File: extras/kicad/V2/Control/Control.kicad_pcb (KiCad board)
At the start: 2 copper layers, 181.3 x 110 mm, 45 parts, among them J1 Ultrasonic Ranging, J2 Conn_01x05, J3 Output, J4 Input, J6 left, J7 right, P8 BeagleBone_Black_Header, P9 BeagleBone_Black_Header, U1 SparkFun-micromod, U2 MPU-6050, U4 BNO085-breackout, U5 TJA1042T-3, U6 PCA9557PW

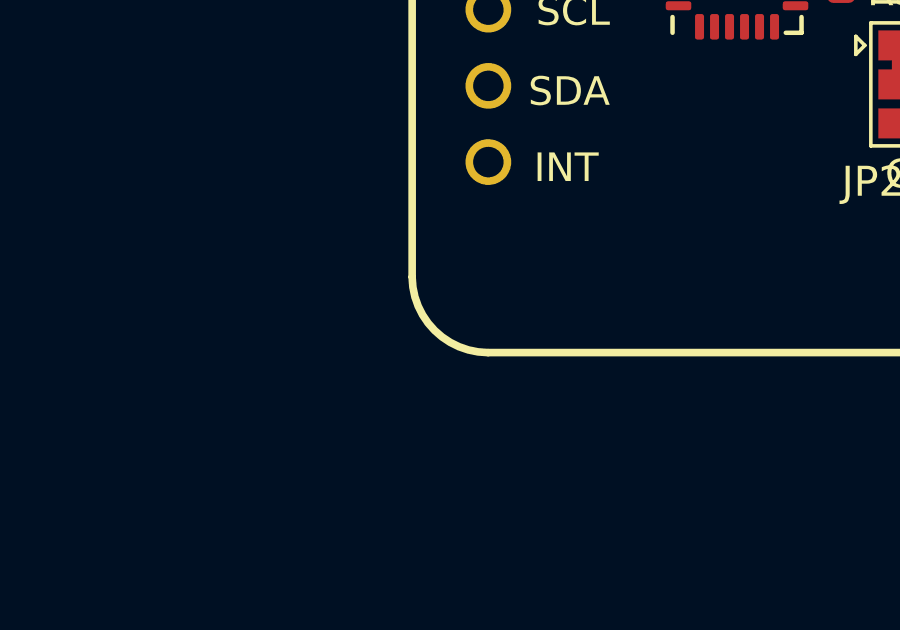
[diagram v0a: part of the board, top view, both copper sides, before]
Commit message: f
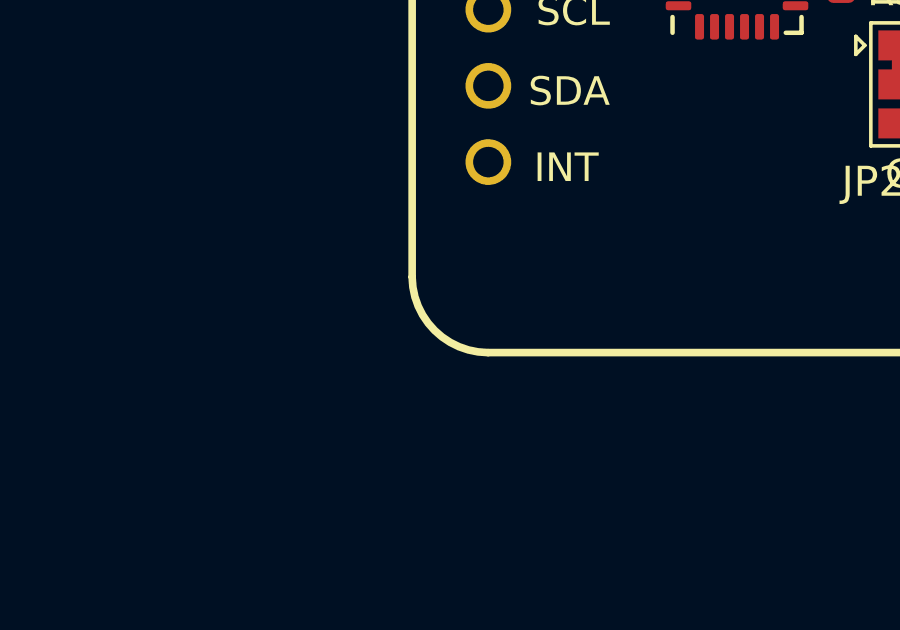
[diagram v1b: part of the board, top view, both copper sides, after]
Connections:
- J6 pad 21: +3V3 -> GND
- J6 pad 33: +3V3 -> GND
- J7 pad 32: +3V3 -> GND
- J7 pad 40: +3V3 -> GND
- P9 pad 17: /GPIO[4] -> SPI_CS
- U1 pad 55: SCL -> SPI_CS
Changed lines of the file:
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@@
   (net 169 "/GPIO[48]")
   (net 170 "/GPIO[51]")
-  (net 171 "/GPIO[4]")
+  (net 171 "SPI_CS")
   (net 172 "/GPIO[5]")
   (net 173 "unconnected-(U6-Pad10)")
@@
       (net 17 "/yellow_1") (pinfunction "AUD_IN") (pintype "input"))
     (pad "55" smd rect (at 4.25 -3.97) (size 0.3 2) (layers "F.Cu" "F.Paste" "F.Mask")
-      (net 2 "SCL") (pinfunction "SPI_CS") (pintype "input"))
+      (net 171 "SPI_CS") (pinfunction "SPI_CS") (pintype "input"))
     (pad "56" smd rect (at 4.5 3.98) (size 0.3 2) (layers "F.Cu" "F.Paste" "F.Mask")
       (net 19 "/Green_1") (pinfunction "AUD_OUT") (pintype "input"))
@@
       (net 1 "GND") (pinfunction "Pin_20") (pintype "passive"))
     (pad "21" thru_hole oval (at 0 25.4 90) (size 1.7 1.7) (drill 1) (layers F&B.Cu *.Mask)
-      (net 4 "+3V3") (pinfunction "Pin_21") (pintype "passive"))
+      (net 1 "GND") (pinfunction "Pin_21") (pintype "passive"))
     (pad "22" thru_hole oval (at 2.54 25.4 90) (size 1.7 1.7) (drill 1) (layers F&B.Cu *.Mask)
       (net 14 "unconnected-(J6-Pad22)") (pinfunction "Pin_22") (pintype "passive"))
@@
       (net 1 "GND") (pinfunction "Pin_32") (pintype "passive"))
     (pad "33" thru_hole oval (at 0 40.64 90) (size 1.7 1.7) (drill 1) (layers F&B.Cu *.Mask)
-      (net 4 "+3V3") (pinfunction "Pin_33") (pintype "passive"))
+      (net 1 "GND") (pinfunction "Pin_33") (pintype "passive"))
     (pad "34" thru_hole oval (at 2.54 40.64 90) (size 1.7 1.7) (drill 1) (layers F&B.Cu *.Mask)
       (net 23 "BIN1_1") (pinfunction "Pin_34") (pintype "passive"))
@@
       (net 1 "GND") (pinfunction "Pin_31") (pintype "passive"))
     (pad "32" thru_hole oval (at 2.54 38.1 90) (size 1.7 1.7) (drill 1) (layers F&B.Cu *.Mask)
-      (net 4 "+3V3") (pinfunction "Pin_32") (pintype "passive"))
+      (net 1 "GND") (pinfunction "Pin_32") (pintype "passive"))
     (pad "33" thru_hole oval (at 0 40.64 90) (size 1.7 1.7) (drill 1) (layers F&B.Cu *.Mask)
       (net 50 "unconnected-(J7-Pad33)") (pinfunction "Pin_33") (pintype "passive"))
@@
       (net 55 "unconnected-(J7-Pad39)") (pinfunction "Pin_39") (pintype "passive"))
     (pad "40" thru_hole oval (at 2.54 48.26 90) (size 1.7 1.7) (drill 1) (layers F&B.Cu *.Mask)
-      (net 4 "+3V3") (pinfunction "Pin_40") (pintype "passive"))
+      (net 1 "GND") (pinfunction "Pin_40") (pintype "passive"))
     (model "${KICAD6_3DMODEL_DIR}/Connector_PinHeader_2.54mm.3dshapes/PinHeader_2x20_P2.54mm_Vertical.wrl"
       (offset (xyz 0 0 0))
@@
     (descr "24-Lead Plastic QFN (4mm x 4mm); Pitch 0.5mm; EP 2.7x2.6mm; for InvenSense motion sensors; keepout area marked (Package see: https://store.invensense.com/datasheets/invensense/MPU-6050_DataSheet_V3%204.pdf; See also https://www.invensense.com/wp-content/uploads/2015/02/InvenSense-MEMS-Handling.pdf)")
     (tags "QFN 0.5")
+    (property "LCSC" "C50278")
     (property "Sheetfile" "Control.kicad_sch")
     (property "Sheetname" "")
@@
     (fp_arc (start 10.883614 -12.0415) (mid 12.657311 -11.285145) (end 13.388855 -9.501066) (layer "F.SilkS") (width 0.254))
     (fp_arc (start -12.011386 -9.5015) (mid -11.267437 -11.297551) (end -9.471386 -12.0415) (layer "F.SilkS") (width 0.254))
-    (fp_arc (start 13.389614 8.2945) (mid 12.651813 10.068874) (end 10.882752 10.819321) (layer "F.SilkS") (width 0.254))
+    (fp_arc (start 13.389614 8.2945) (mid 12.651812 10.06887) (end 10.882752 10.819321) (layer "F.SilkS") (width 0.254))
     (fp_arc (start -9.505386 10.8185) (mid -11.279706 10.062522) (end -12.011614 8.278139) (layer "F.SilkS") (width 0.254))
     (fp_line (start 13.388614 10.8185) (end -12.011386 10.8185) (layer "F.CrtYd") (width 0.152))
@@
       (net 170 "/GPIO[51]") (pinfunction "Pin_16") (pintype "passive"))
     (pad "17" thru_hole oval locked (at 0 -20.32 270) (size 1.7 1.7) (drill 1) (layers F&B.Cu *.Mask)
-      (net 171 "/GPIO[4]") (pinfunction "Pin_17") (pintype "passive"))
+      (net 171 "SPI_CS") (pinfunction "Pin_17") (pintype "passive"))
     (pad "18" thru_hole oval locked (at 2.54 -20.32 270) (size 1.7 1.7) (drill 1) (layers F&B.Cu *.Mask)
       (net 172 "/GPIO[5]") (pinfunction "Pin_18") (pintype "passive"))

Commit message: g
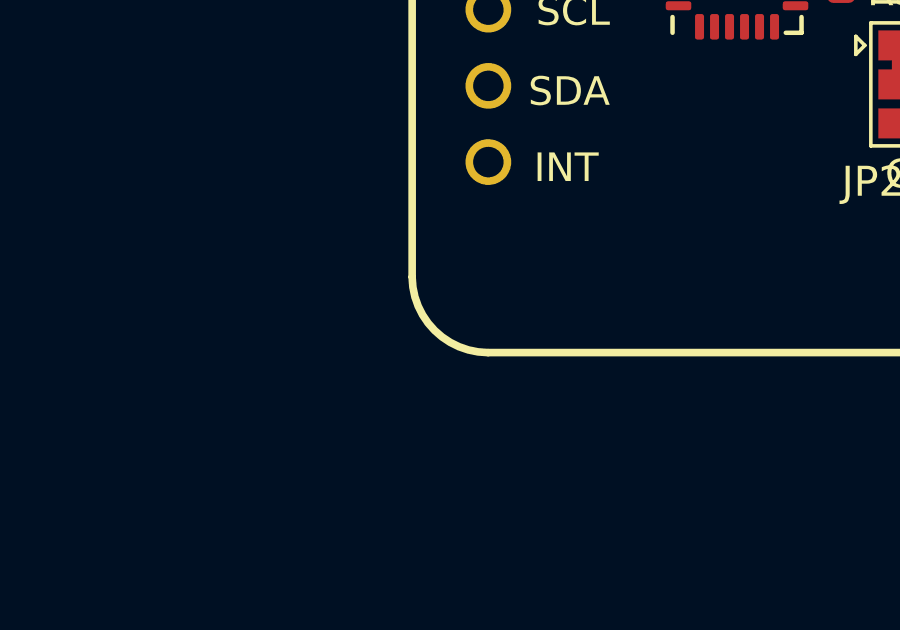
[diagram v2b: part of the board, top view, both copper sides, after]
